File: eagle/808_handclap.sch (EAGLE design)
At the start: 82 parts, among them IC1 LM339N, Q1 2N3906, Q2 2N3904, Q3 2N3906, Q4 2N3906, Q5 2N3904, Q6 2N3904, Q7 2N3904, U1 POWER, U19 µPC4558C, U21 µPC4558C, U22 BA6110SIL

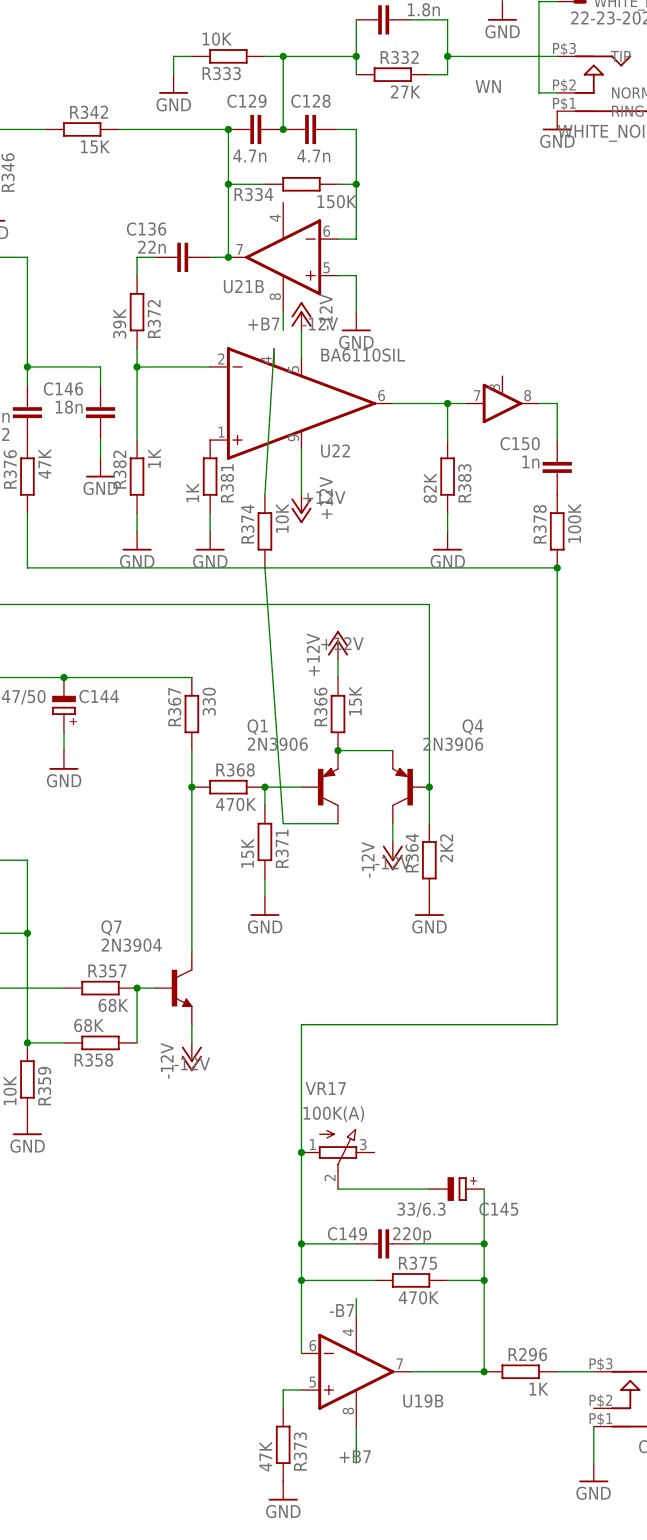
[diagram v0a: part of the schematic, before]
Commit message: opamps
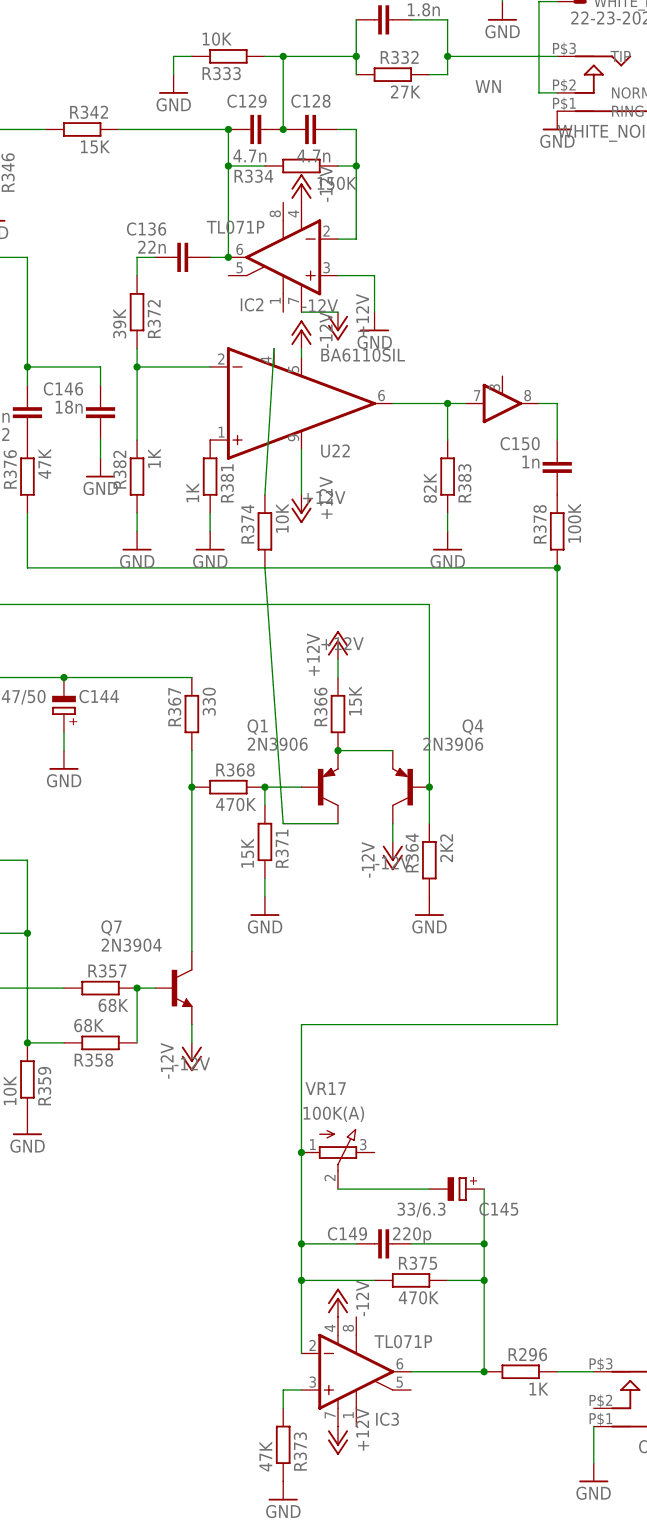
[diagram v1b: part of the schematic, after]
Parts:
- removed U19, U21: µPC4558C, TR808clone:µPC4558C
- added IC2, IC3: TL071P, 808_lt:TL071P
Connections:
- removed net +B7: U19G$3.V+, U21G$3.V+
- removed net -B7: U19G$3.V-
- net +12V: now also IC2.V+, IC3.V+
- net -12V: now also IC2.V-, IC3.V-
- net GND: now also IC2.+IN; no longer U21B.+IN
- net N$10: now also IC2.OUT; no longer U21B.OUT
- net N$54: now also IC2.-IN; no longer U21B.-IN
- net N$91: now also IC3.+IN; no longer U19B.+IN
- net N$92: now also IC3.-IN; no longer U19B.-IN
- net N$97: now also IC3.OUT; no longer U19B.OUT
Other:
- moved on the sheet: R334
